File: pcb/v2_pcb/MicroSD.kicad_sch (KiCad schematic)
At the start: 9 parts, among them J3 DM3CS-SF

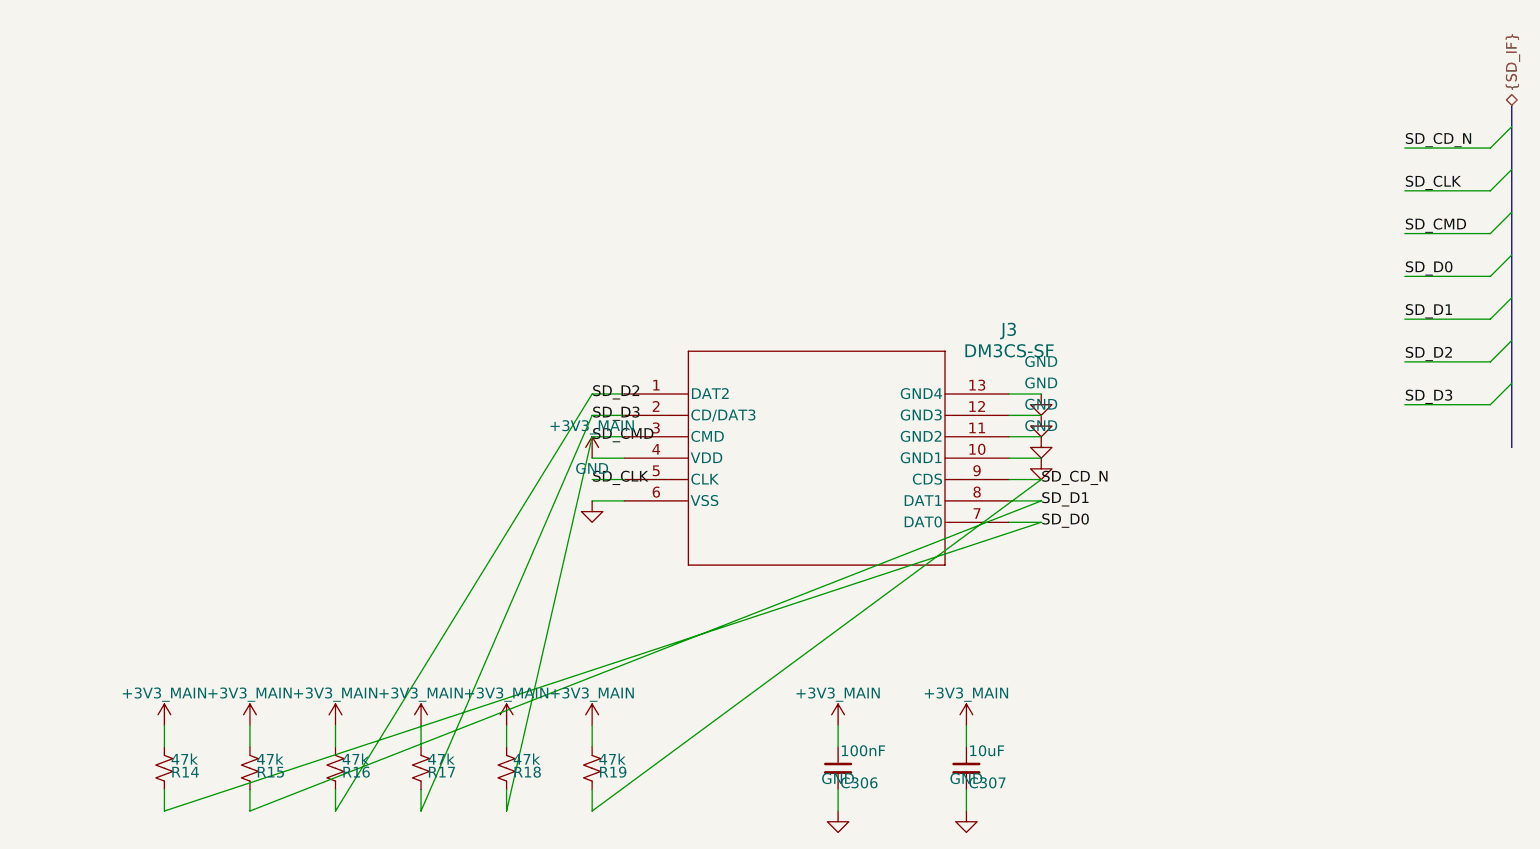
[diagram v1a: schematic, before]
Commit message: clean pcb
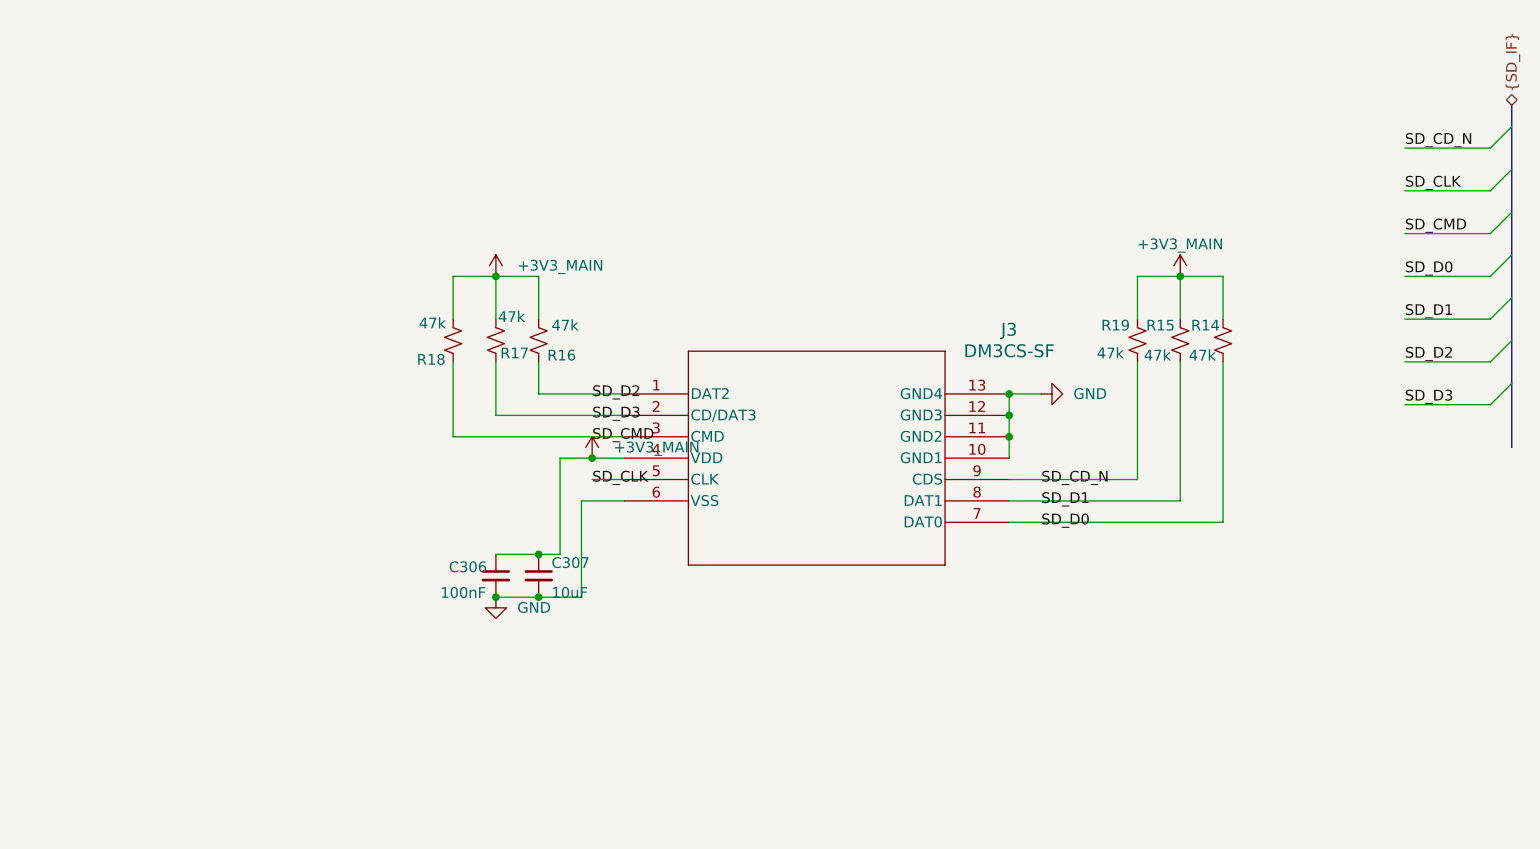
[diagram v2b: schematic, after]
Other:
- moved on the sheet: C306, C307, R14, R15, R16, R17, R18, R19

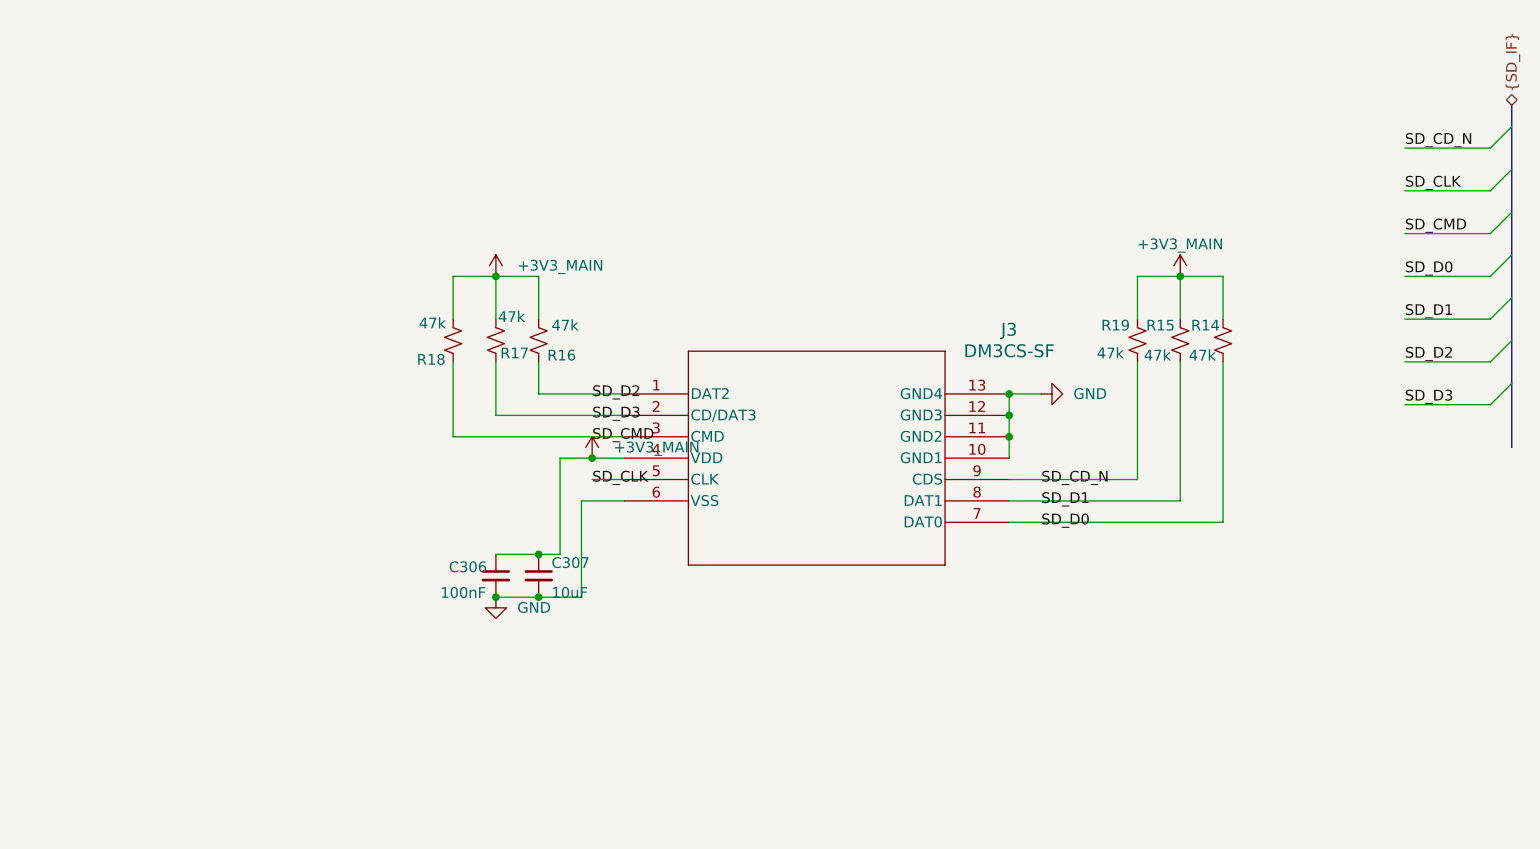
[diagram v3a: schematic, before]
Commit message: minor fixes
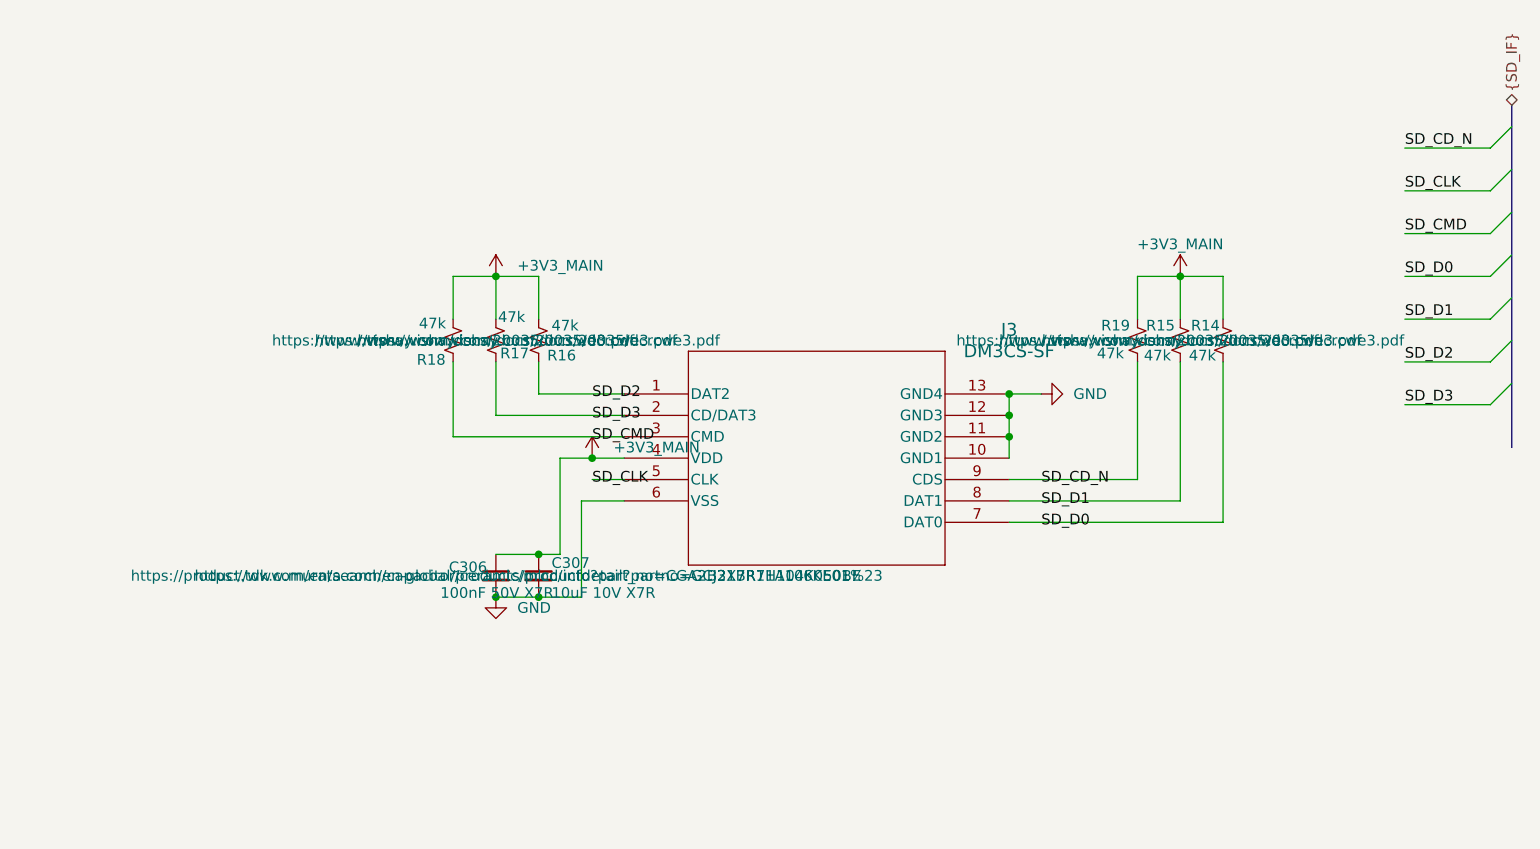
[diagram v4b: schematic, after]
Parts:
- C306: value 100nF -> 100nF 50V X7R; Dielectric (none) -> X7R; MPN (none) -> CGA2B3X7R1H104K050BE; Manufacturer (none) -> TDK; Qualification (none) -> AEC-Q200; Termination (none) -> Soft termination; Tolerance (none) -> ±10%; Voltage (none) -> 50 VDC
- C307: value 10uF -> 10uF 10V X7R; Dielectric (none) -> X7R; MPN (none) -> GCJ21BR71A106KE01L; Manufacturer (none) -> Murata; Qualification (none) -> AEC-Q200; Termination (none) -> Soft termination; Tolerance (none) -> ±10%; Voltage (none) -> 10 VDC
- R14, R15, R16, R17, R18, R19: MPN (none) -> CRCW040247K0FKED; Manufacturer (none) -> Vishay; Power (none) -> 0.063 W; TCR (none) -> ±100 ppm/K; Tolerance (none) -> ±1%
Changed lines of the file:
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@@
 			)
 		)
-		(property "Datasheet" ""
+		(property "Datasheet" "https://www.vishay.com/docs/20035/dcrcwe3.pdf"
 			(at 109.22 83.82 0)
 			(show_name no)
@@
 			)
 		)
+    (property "Manufacturer" "Vishay" (at 109.22 83.82 0)
+      (effects (font (size 1.27 1.27)) (hide yes))
+    )
+    (property "MPN" "CRCW040247K0FKED" (at 109.22 83.82 0)
+      (effects (font (size 1.27 1.27)) (hide yes))
+    )
+    (property "Tolerance" "±1%" (at 109.22 83.82 0)
+      (effects (font (size 1.27 1.27)) (hide yes))
+    )
+    (property "Power" "0.063 W" (at 109.22 83.82 0)
+      (effects (font (size 1.27 1.27)) (hide yes))
+    )
+    (property "TCR" "±100 ppm/K" (at 109.22 83.82 0)
+      (effects (font (size 1.27 1.27)) (hide yes))
+    )
 		(pin "1"
 		)
@@
 			)
 		)
-		(property "Datasheet" "DM3CS-SF"
+		(property "Datasheet" "https://www.hirose.com/product/download/?distributor=all&lang=en&num=DM3CS-SF&type=specSheet"
 			(at 142.24 92.71 0)
 			(hide yes)
@@
 			)
 		)
-		(property "Description" ""
+		(property "Description" "Hirose DM3CS-SF hinged push-pull microSD socket"
 			(at 142.24 92.71 0)
 			(hide yes)
@@
 			)
 		)
-		(property "Value" "100nF"
+		(property "Value" "100nF 50V X7R"
 			(at 97.536 113.792 0)
 			(show_name no)
@@
 			)
 		)
-		(property "Datasheet" ""
+		(property "Datasheet" "https://product.tdk.com/en/search/capacitor/ceramic/mlcc/info?part_no=CGA2B3X7R1H104K050BE"
 			(at 104.14 111.76 0)
 			(show_name no)
@@
 			)
 		)
+    (property "Manufacturer" "TDK" (at 104.14 111.76 0)
+      (effects (font (size 1.27 1.27)) (hide yes))
+    )
+    (property "MPN" "CGA2B3X7R1H104K050BE" (at 104.14 111.76 0)
+      (effects (font (size 1.27 1.27)) (hide yes))
+    )
+    (property "Voltage" "50 VDC" (at 104.14 111.76 0)
+      (effects (font (size 1.27 1.27)) (hide yes))
+    )
+    (property "Tolerance" "±10%" (at 104.14 111.76 0)
+      (effects (font (size 1.27 1.27)) (hide yes))
+    )
+    (property "Dielectric" "X7R" (at 104.14 111.76 0)
+      (effects (font (size 1.27 1.27)) (hide yes))
+    )
+    (property "Qualification" "AEC-Q200" (at 104.14 111.76 0)
+      (effects (font (size 1.27 1.27)) (hide yes))
+    )
+    (property "Termination" "Soft termination" (at 104.14 111.76 0)
+      (effects (font (size 1.27 1.27)) (hide yes))
+    )
 		(pin "1"
 		)
@@
 			)
 		)
-		(property "Datasheet" ""
+		(property "Datasheet" "https://www.vishay.com/docs/20035/dcrcwe3.pdf"
 			(at 180.34 83.82 0)
 			(show_name no)
@@
 			)
 		)
+    (property "Manufacturer" "Vishay" (at 180.34 83.82 0)
+      (effects (font (size 1.27 1.27)) (hide yes))
+    )
+    (property "MPN" "CRCW040247K0FKED" (at 180.34 83.82 0)
+      (effects (font (size 1.27 1.27)) (hide yes))
+    )
+    (property "Tolerance" "±1%" (at 180.34 83.82 0)
+      (effects (font (size 1.27 1.27)) (hide yes))
+    )
+    (property "Power" "0.063 W" (at 180.34 83.82 0)
+      (effects (font (size 1.27 1.27)) (hide yes))
+    )
+    (property "TCR" "±100 ppm/K" (at 180.34 83.82 0)
+      (effects (font (size 1.27 1.27)) (hide yes))
+    )
 		(pin "1"
 		)
@@
 			)
 		)
-		(property "Datasheet" ""
+		(property "Datasheet" "https://www.vishay.com/docs/20035/dcrcwe3.pdf"
 			(at 104.14 83.82 0)
 			(show_name no)
@@
 			)
 		)
+    (property "Manufacturer" "Vishay" (at 104.14 83.82 0)
+      (effects (font (size 1.27 1.27)) (hide yes))
+    )
+    (property "MPN" "CRCW040247K0FKED" (at 104.14 83.82 0)
+      (effects (font (size 1.27 1.27)) (hide yes))
+    )
+    (property "Tolerance" "±1%" (at 104.14 83.82 0)
+      (effects (font (size 1.27 1.27)) (hide yes))
+    )
+    (property "Power" "0.063 W" (at 104.14 83.82 0)
+      (effects (font (size 1.27 1.27)) (hide yes))
+    )
+    (property "TCR" "±100 ppm/K" (at 104.14 83.82 0)
+      (effects (font (size 1.27 1.27)) (hide yes))
+    )
 		(pin "1"
 		)
@@
 			)
 		)
-		(property "Datasheet" ""
+		(property "Datasheet" "https://www.vishay.com/docs/20035/dcrcwe3.pdf"
 			(at 190.5 83.82 0)
 			(show_name no)
@@
 			)
 		)
+    (property "Manufacturer" "Vishay" (at 190.5 83.82 0)
+      (effects (font (size 1.27 1.27)) (hide yes))
+    )
+    (property "MPN" "CRCW040247K0FKED" (at 190.5 83.82 0)
+      (effects (font (size 1.27 1.27)) (hide yes))
+    )
+    (property "Tolerance" "±1%" (at 190.5 83.82 0)
+      (effects (font (size 1.27 1.27)) (hide yes))
+    )
+    (property "Power" "0.063 W" (at 190.5 83.82 0)
+      (effects (font (size 1.27 1.27)) (hide yes))
+    )
+    (property "TCR" "±100 ppm/K" (at 190.5 83.82 0)
+      (effects (font (size 1.27 1.27)) (hide yes))
+    )
 		(pin "1"
 		)
@@
 			)
 		)
-		(property "Datasheet" ""
+		(property "Datasheet" "https://www.vishay.com/docs/20035/dcrcwe3.pdf"
 			(at 99.06 83.82 0)
 			(show_name no)
@@
 			)
 		)
+    (property "Manufacturer" "Vishay" (at 99.06 83.82 0)
+      (effects (font (size 1.27 1.27)) (hide yes))
+    )
+    (property "MPN" "CRCW040247K0FKED" (at 99.06 83.82 0)
+      (effects (font (size 1.27 1.27)) (hide yes))
+    )
+    (property "Tolerance" "±1%" (at 99.06 83.82 0)
+      (effects (font (size 1.27 1.27)) (hide yes))
+    )
+    (property "Power" "0.063 W" (at 99.06 83.82 0)
+      (effects (font (size 1.27 1.27)) (hide yes))
+    )
+    (property "TCR" "±100 ppm/K" (at 99.06 83.82 0)
+      (effects (font (size 1.27 1.27)) (hide yes))
+    )
 		(pin "1"
 		)
@@
 			)
 		)
-		(property "Datasheet" ""
+		(property "Datasheet" "https://www.vishay.com/docs/20035/dcrcwe3.pdf"
 			(at 185.42 83.82 0)
 			(show_name no)
@@
 			)
 		)
+    (property "Manufacturer" "Vishay" (at 185.42 83.82 0)
+      (effects (font (size 1.27 1.27)) (hide yes))
+    )
+    (property "MPN" "CRCW040247K0FKED" (at 185.42 83.82 0)
+      (effects (font (size 1.27 1.27)) (hide yes))
+    )
+    (property "Tolerance" "±1%" (at 185.42 83.82 0)
+      (effects (font (size 1.27 1.27)) (hide yes))
+    )
+    (property "Power" "0.063 W" (at 185.42 83.82 0)
+      (effects (font (size 1.27 1.27)) (hide yes))
+    )
+    (property "TCR" "±100 ppm/K" (at 185.42 83.82 0)
+      (effects (font (size 1.27 1.27)) (hide yes))
+    )
 		(pin "1"
 		)
@@
 			)
 		)
-		(property "Value" "10uF"
+		(property "Value" "10uF 10V X7R"
 			(at 110.744 113.792 0)
 			(show_name no)
@@
 			)
 		)
-		(property "Datasheet" ""
+		(property "Datasheet" "https://www.murata.com/en-global/products/productdetail?partno=GCJ21BR71A106KE01%23"
 			(at 109.22 111.76 0)
 			(show_name no)
@@
 			)
 		)
-		(pin "1"
-		)
+    (property "Manufacturer" "Murata" (at 109.22 111.76 0)
+      (effects (font (size 1.27 1.27)) (hide yes))
+    )
+    (property "MPN" "GCJ21BR71A106KE01L" (at 109.22 111.76 0)
+      (effects (font (size 1.27 1.27)) (hide yes))
+    )
+    (property "Voltage" "10 VDC" (at 109.22 111.76 0)
+      (effects (font (size 1.27 1.27)) (hide yes))
+    )
+    (property "Tolerance" "±10%" (at 109.22 111.76 0)
+      (effects (font (size 1.27 1.27)) (hide yes))
+    )
+    (property "Dielectric" "X7R" (at 109.22 111.76 0)
+      (effects (font (size 1.27 1.27)) (hide yes))
+    )
+    (property "Termination" "Soft termination" (at 109.22 111.76 0)
+      (effects (font (size 1.27 1.27)) (hide yes))
+    )
+    (property "Qualification" "AEC-Q200" (at 109.22 111.76 0)
+      (effects (font (size 1.27 1.27)) (hide yes))
+    )
+		(pin "1"
+		)
